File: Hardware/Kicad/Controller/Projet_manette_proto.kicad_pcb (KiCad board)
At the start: 2 copper layers, 67 parts, among them J1 Conn_01x02, SW1 SW_Push, SW10 SW_Push, SW11 SW_DIP_x01, SW12 SW_Push, SW13 SW_DIP_x01, SW2 SW_Push, SW3 SW_Push, SW4 SW_Push, SW5 SW_Push, SW6 SW_Push, SW7 SW_Push, SW8 SW_Push, SW9 SW_Push, U1 STM32L412KBTx, U2 MIC5219-3.3YMM, U3 NRF24L01, Y1 16MHz

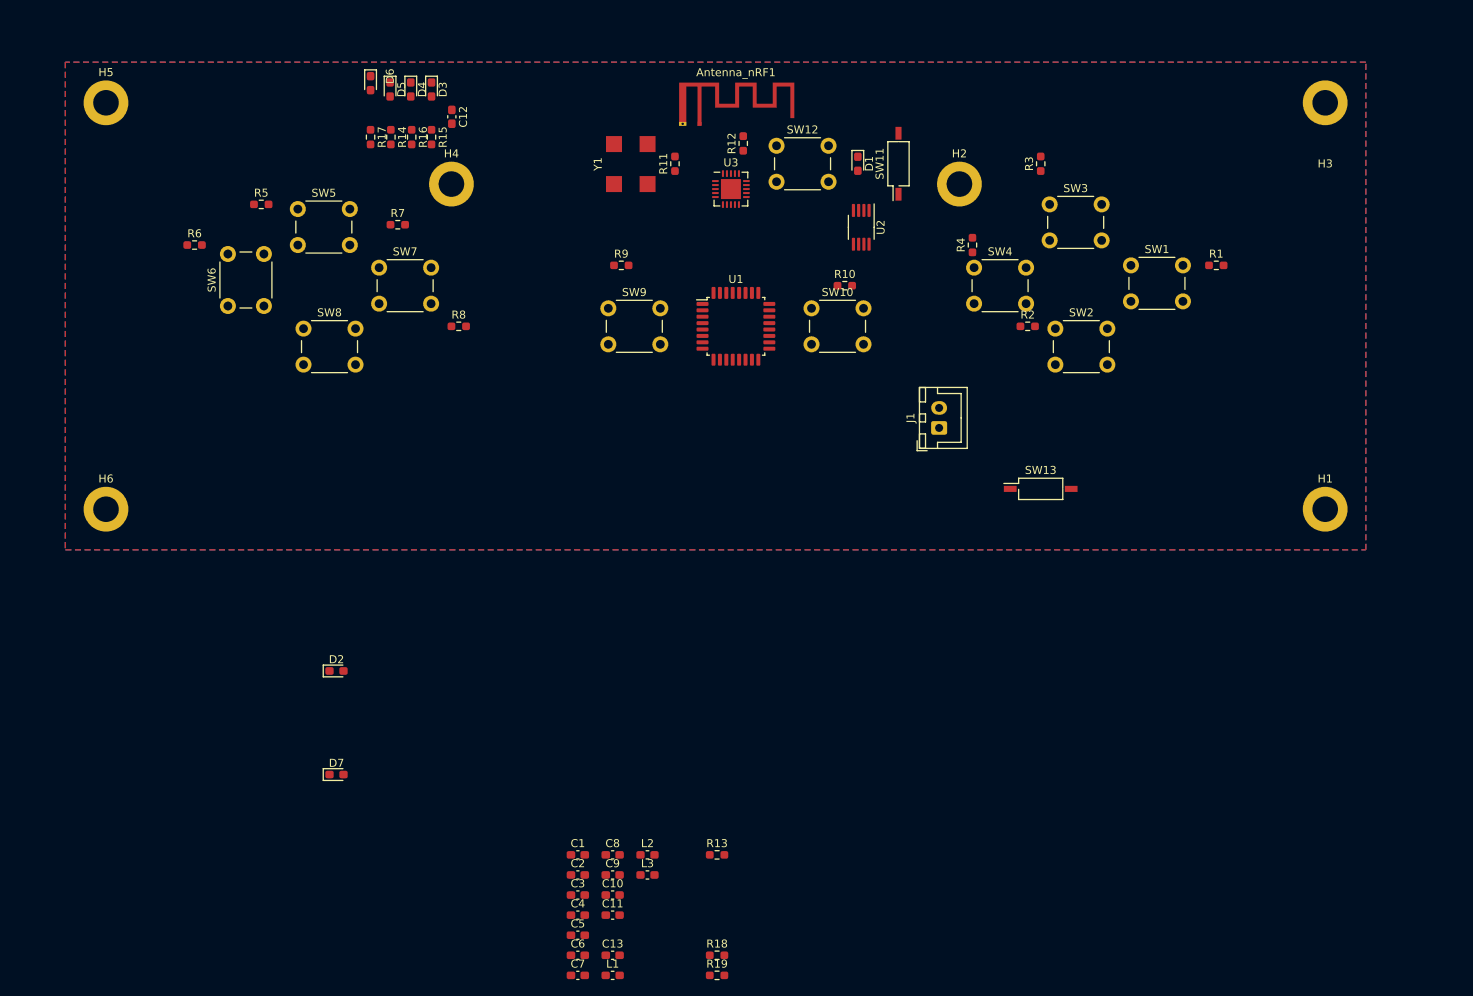
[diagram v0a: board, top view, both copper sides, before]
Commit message: CONTROLER V1
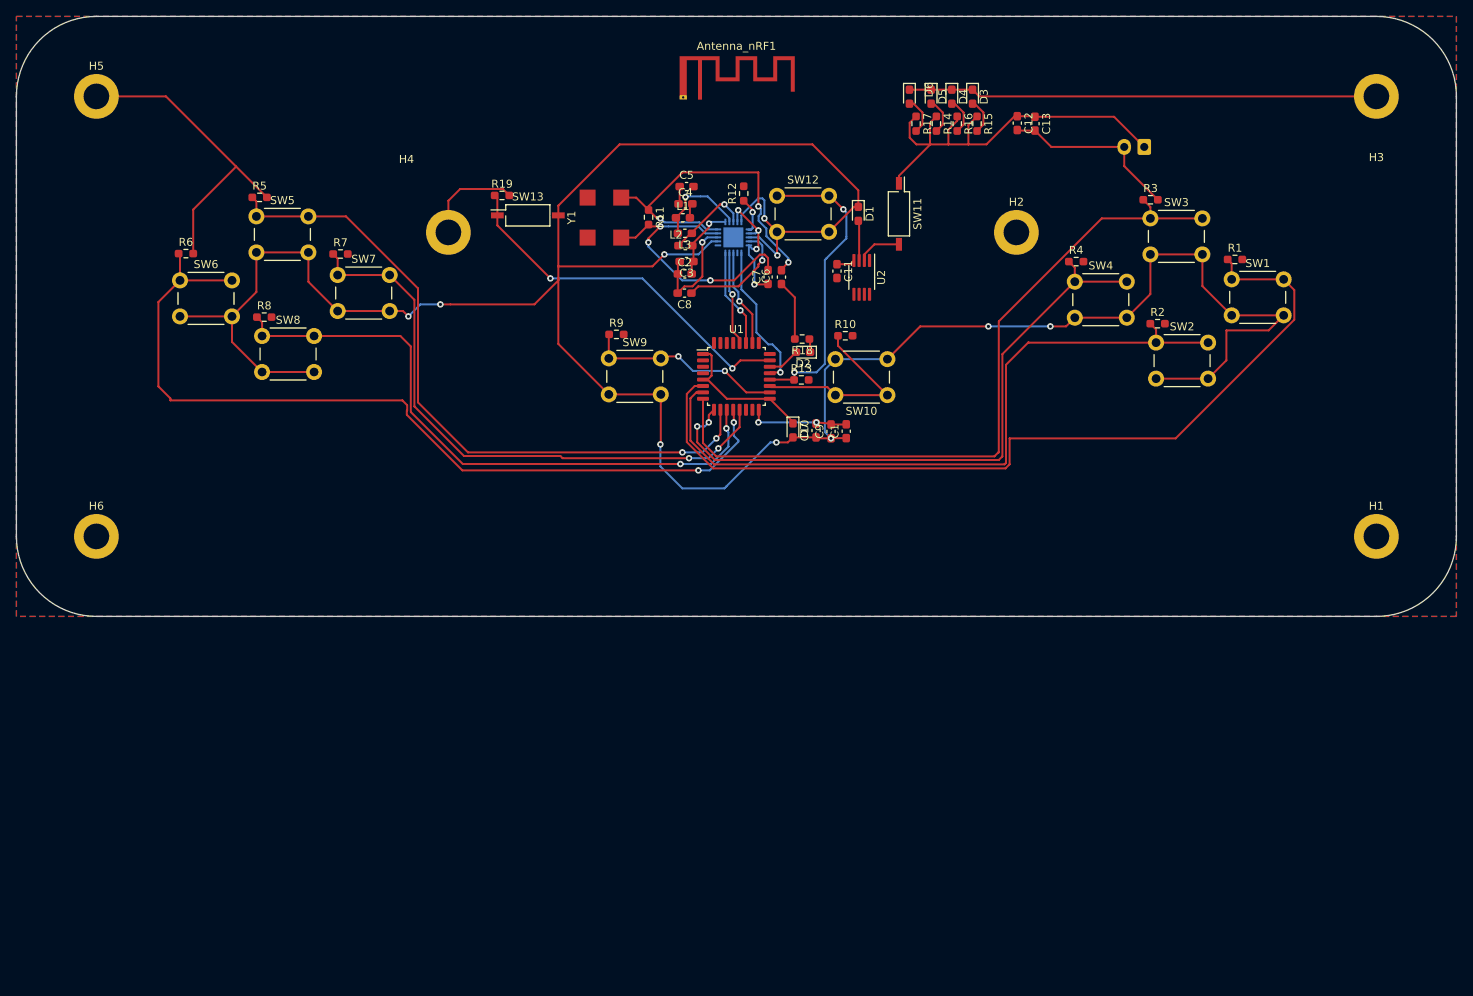
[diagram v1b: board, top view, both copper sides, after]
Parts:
- J1, U3: moved to B.Cu
- moved C13 116.6 mm to (192.3, 53.4), turned to -90 degrees
- moved R19 101.1 mm to (125.7, 62.4)
- moved L1 95.1 mm to (148.3, 65.2)
- moved C5 94.6 mm to (148.8, 61.3)
- moved C7 90.5 mm to (159.0, 72.6), turned to 90 degrees
- moved C4 89.9 mm to (148.6, 63.4)
- moved C6 88.5 mm to (160.6, 72.6), turned to 90 degrees
- moved C11 85.2 mm to (167.6, 71.8), turned to -90 degrees
- moved C3 80.3 mm to (148.8, 70.6), turned to 180 degrees
- moved L3 80.3 mm to (148.6, 67.1), turned to 180 degrees
- moved R18 77.8 mm to (163.2, 80.3), turned to 180 degrees
- moved C2 76.3 mm to (148.6, 72.2)
- moved L2 76.3 mm to (148.6, 68.7)
- moved SW13 72.7 mm to (128.9, 64.9)
- moved D7 71.5 mm to (162.1, 91.7), turned to -90 degrees
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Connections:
- Antenna_nRF1 pad 2: A_Button -> GND
- C1 pad 2: A_Button -> GND
- C10 pad 2: A_Button -> GND
- C11 pad 2: A_Button -> GND
- C12 pad 2: A_Button -> GND
- C13 pad 2: A_Button -> GND
- C2 pad 1: A_Button -> GND
- C3 pad 2: A_Button -> GND
- C5 pad 2: A_Button -> GND
- C6 pad 1: A_Button -> GND
- C7 pad 1: A_Button -> GND
- C8 pad 2: A_Button -> GND
- C9 pad 2: A_Button -> GND
- D3 pad 1: A_Button -> GND
- D4 pad 1: A_Button -> GND
- D5 pad 1: A_Button -> GND
- D6 pad 1: A_Button -> GND
- H1 pad 1: A_Button -> GND
- H2 pad 1: A_Button -> GND
- H3 pad 1: A_Button -> GND
- H4 pad 1: A_Button -> GND
- H5 pad 1: A_Button -> GND
- H6 pad 1: A_Button -> GND
- J1 pad 2: A_Button -> GND
- R1 pad 1: Net-(R1-Pad1) -> A_Button
- R1 pad 2: A_Button -> GND
- R10 pad 1: Net-(R10-Pad1) -> SE_Button
- R10 pad 2: A_Button -> GND
- R12 pad 2: A_Button -> GND
- R13 pad 2: A_Button -> GND
- R18 pad 2: A_Button -> GND
- R19 pad 1: Net-(R19-Pad1) -> NES/SNES_switcher
- R19 pad 2: A_Button -> GND
- R2 pad 1: Net-(R2-Pad1) -> B_Button
- R2 pad 2: A_Button -> GND
- R3 pad 1: Net-(R3-Pad1) -> X_Button
- R3 pad 2: A_Button -> GND
- R4 pad 1: Net-(R4-Pad1) -> Y_Button
- R4 pad 2: A_Button -> GND
- R5 pad 1: Net-(R5-Pad1) -> UC_Button
- R5 pad 2: A_Button -> GND
- R6 pad 1: Net-(R6-Pad1) -> LC_Button
- R6 pad 2: A_Button -> GND
- R7 pad 1: Net-(R7-Pad1) -> RC_Button
- R7 pad 2: A_Button -> GND
- R8 pad 1: Net-(R8-Pad1) -> DC_Button
- R8 pad 2: A_Button -> GND
- R9 pad 1: Net-(R9-Pad1) -> ST_Button
- R9 pad 2: A_Button -> GND
- SW1 pad 1: Net-(R1-Pad1) -> A_Button
- SW10 pad 1: Net-(R10-Pad1) -> SE_Button
- SW13 pad 1: Net-(R19-Pad1) -> NES/SNES_switcher
- SW2 pad 1: Net-(R2-Pad1) -> B_Button
- SW3 pad 1: Net-(R3-Pad1) -> X_Button
- SW4 pad 1: Net-(R4-Pad1) -> Y_Button
- SW5 pad 1: Net-(R5-Pad1) -> UC_Button
- SW6 pad 1: Net-(R6-Pad1) -> LC_Button
- SW7 pad 1: Net-(R7-Pad1) -> RC_Button
- SW8 pad 1: Net-(R8-Pad1) -> DC_Button
- SW9 pad 1: Net-(R9-Pad1) -> ST_Button
- U1 pad 10: A_Button -> UC_Button
- U1 pad 11: A_Button -> DC_Button
- U1 pad 12: A_Button -> LC_Button
- U1 pad 13: A_Button -> RC_Button
- U1 pad 16: A_Button -> GND
- U1 pad 18: A_Button -> ST_Button
- U1 pad 19: A_Button -> SE_Button
- U1 pad 23: A_Button -> NES/SNES_switcher
- U1 pad 32: A_Button -> GND
- U1 pad 7: A_Button -> B_Button
- U1 pad 8: A_Button -> X_Button
- U1 pad 9: A_Button -> Y_Button
- U2 pad 5: A_Button -> GND
- U2 pad 6: A_Button -> GND
- U2 pad 7: A_Button -> GND
- U2 pad 8: A_Button -> GND
- U3 pad 14: A_Button -> GND
- U3 pad 17: A_Button -> GND
- U3 pad 20: A_Button -> GND
- U3 pad 8: A_Button -> GND
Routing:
- net Glob_Alim: track 0.00 -> 341.4 mm, vias 0 -> 11
- net GND: track 0.00 -> 185.2 mm, vias 0 -> 7
- net A_Button: track 0.00 -> 110.1 mm
- net LC_Button: track 0.00 -> 107.8 mm, vias 0 -> 2
- net X_Button: track 0.00 -> 93.3 mm
- net B_Button: track 0.00 -> 89.3 mm
- net UC_Button: track 0.00 -> 85.2 mm, vias 0 -> 2
- net Y_Button: track 0.00 -> 79.6 mm, vias 0 -> 2
- net DC_Button: track 0.00 -> 78.3 mm, vias 0 -> 2
- net RC_Button: track 0.00 -> 74.2 mm, vias 0 -> 2
- net Li-ion: track 0.00 -> 54.0 mm
- net NES/SNES_switcher: track 0.00 -> 45.8 mm, vias 0 -> 2
- net Net-(U3-XC1): track 0.00 -> 44.1 mm, vias 0 -> 3
- net Order_Search: track 0.00 -> 37.8 mm, vias 0 -> 2
- net Net-(U3-XC2): track 0.00 -> 36.1 mm, vias 0 -> 3
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- added copper zone on B.Cu, net GND
- added copper zone on F.Cu, net GND
- removed copper zone on B.Cu, net (none)
- removed copper zone on F.Cu, net (none)
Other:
- board outline added: 180 x 75 mm
